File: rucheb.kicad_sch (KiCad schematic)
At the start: 28 parts, among them IC1 CN3791, IC9 FS312F-G, J1 Conn_01x02, Q1 AO3401A, Q8 FS8205

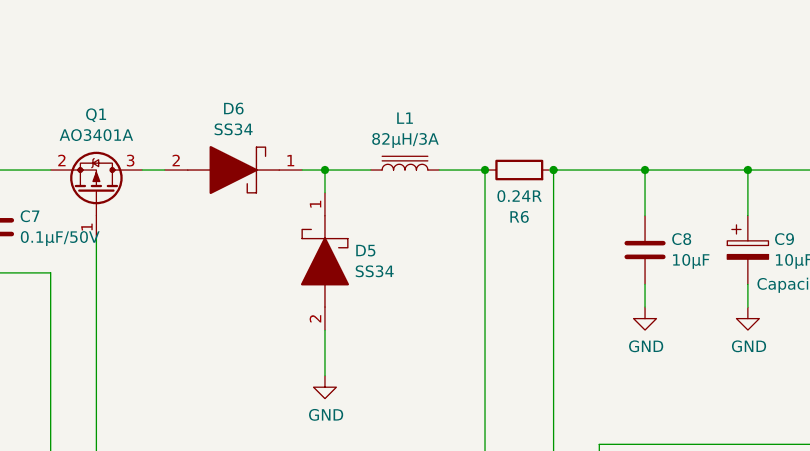
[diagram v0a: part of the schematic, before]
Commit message: update
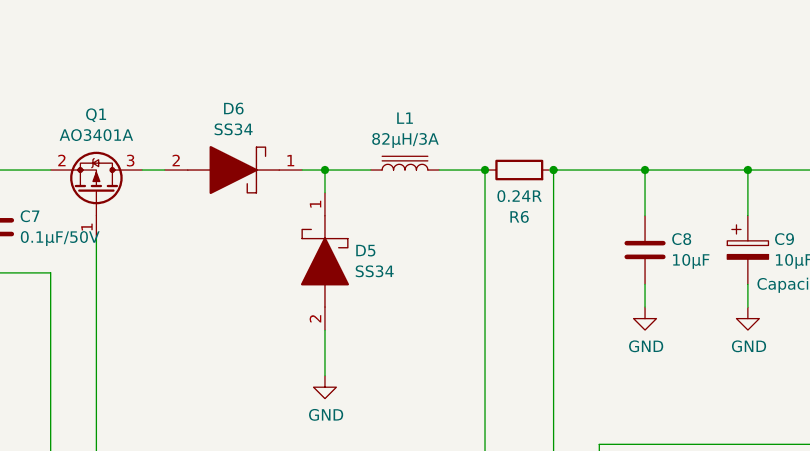
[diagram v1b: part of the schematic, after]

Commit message: Revert "update"
This reverts commit 9afc669c055c7e8087787cb6fdf10dddd7845243.
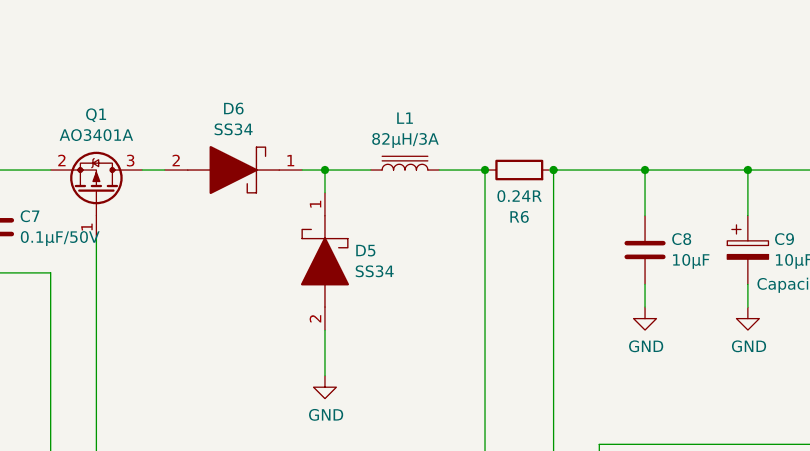
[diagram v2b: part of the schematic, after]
